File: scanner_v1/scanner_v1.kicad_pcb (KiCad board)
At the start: 2 copper layers, 59.3 x 42.2 mm, 47 parts, among them J1 Conn_01x06, J2 Conn_01x03, J3 USB_B, Q1 SS8050, Q2 SS8050, Q3 2N3906, Q4 SS8050, Q5 SS8050, U1 LM321, U2 TS2431BILT, U3 LM321, U4 PIC16F84A-XXSO, U5 LM321, U6 LM321, U7 CH340E, U8 LM7805_TO220, Y1 20Mhz

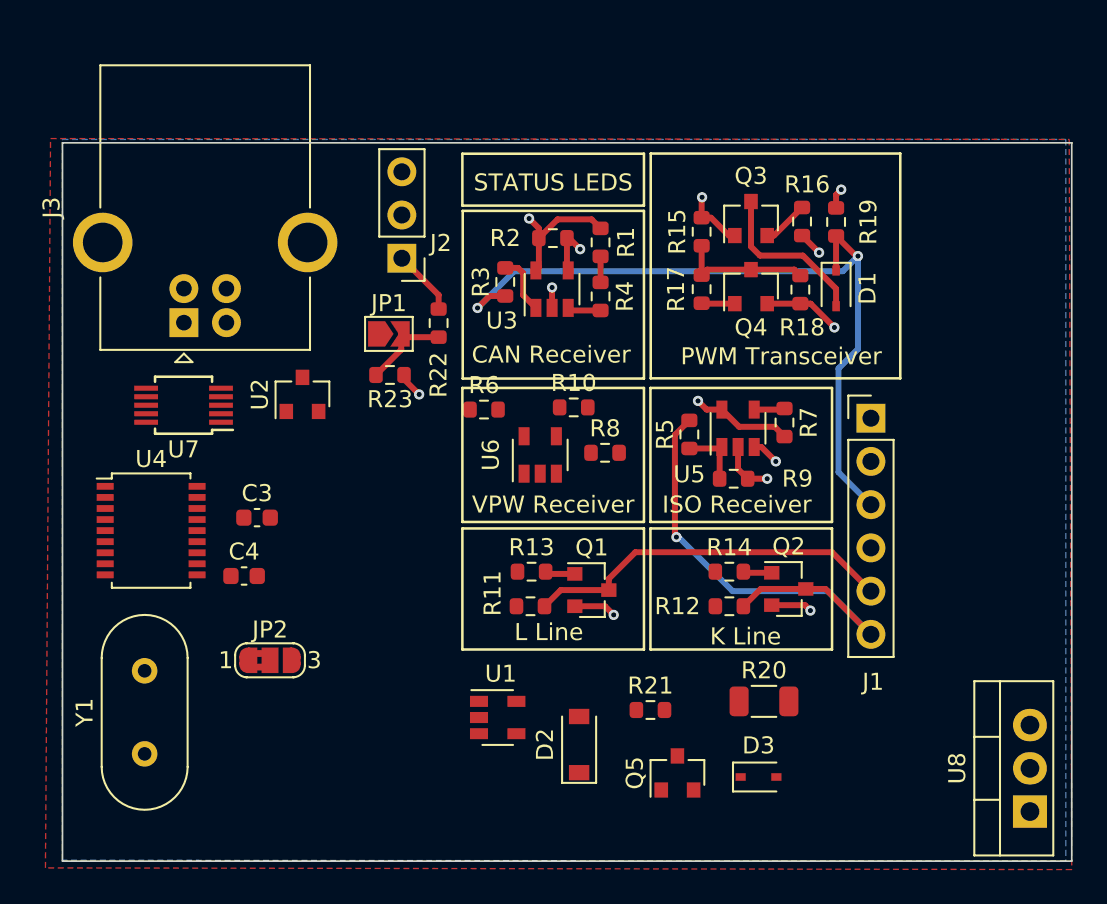
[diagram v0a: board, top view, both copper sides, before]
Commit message: finish v01
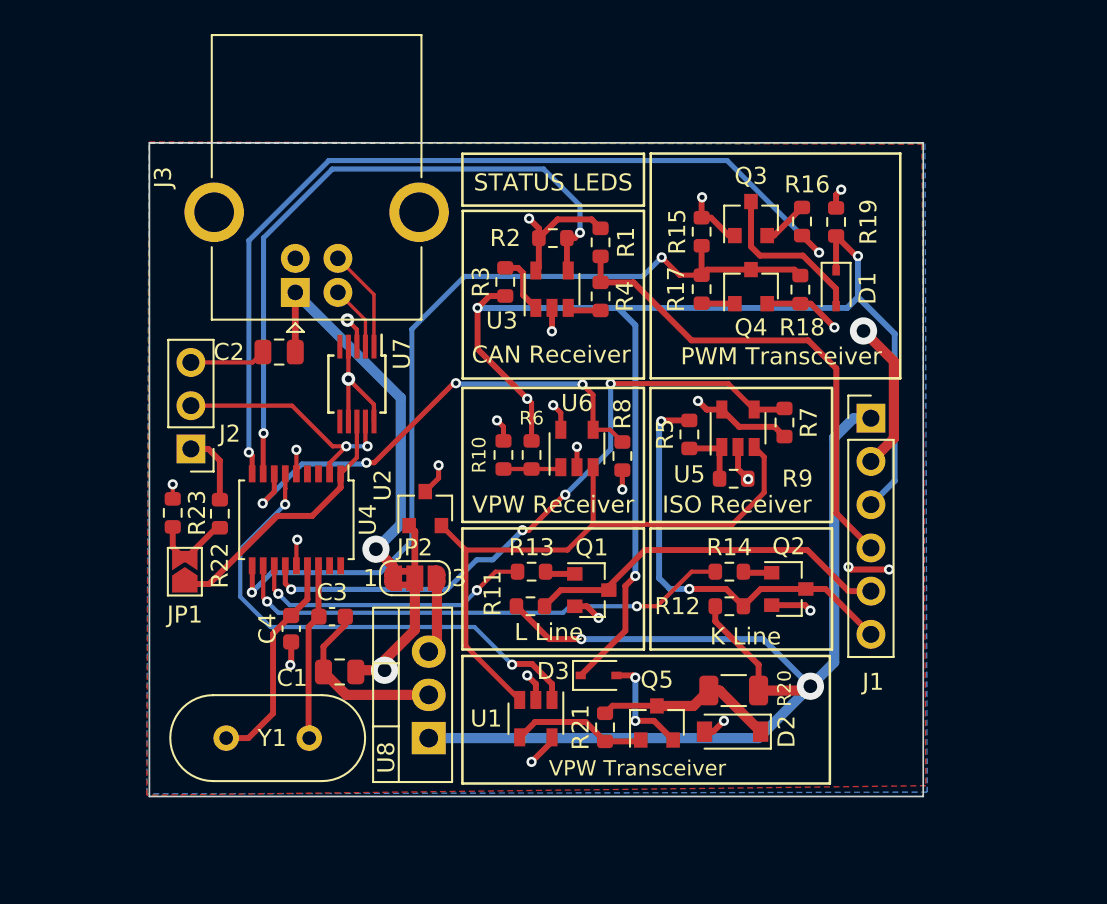
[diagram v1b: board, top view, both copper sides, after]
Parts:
- added C1: 100nF, Capacitor_SMD:C_0805_2012Metric, F.Cu at (129.2, 126.3)
- added C2: 100nF, Capacitor_SMD:C_0805_2012Metric, F.Cu at (125.6, 107.5)
- moved U8 35.6 mm to (134.4, 130.2)
- moved JP1 18.4 mm to (120.1, 120.4), turned to 90 degrees
- moved R22 17.0 mm to (122.1, 117.0)
- moved J2 16.7 mm to (120.4, 113.2)
- moved R23 15.1 mm to (119.4, 116.9), turned to -90 degrees
- moved D3 11.1 mm to (144.4, 126.5)
- moved U7 10.3 mm to (130.2, 109.4), turned to -90 degrees
- moved U2 9.85 mm to (134.2, 116.7)
- moved JP2 9.78 mm to (133.6, 120.8)
- moved D2 9.05 mm to (152.3, 129.8), turned to 180 degrees
- moved U4 8.56 mm to (126.6, 117.3), turned to -90 degrees
- moved C3 7.30 mm to (128.7, 123.0)
- moved J3 6.78 mm to (126.6, 104.0)
- moved R10 4.98 mm to (138.8, 113.5), turned to 90 degrees
- moved Y1 4.88 mm to (122.5, 130.2), turned to 0 degrees
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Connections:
- U1 pad 5: unconnected-(U1-Pad5) -> +5V
- U4 pad 7: /xVPW_T -> /xVPW_R
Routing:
- net +12V: track 0.00 -> 69.9 mm, vias 0 -> 2
- net /xCAN+: track 1.41 -> 52.9 mm, vias 1 -> 2
- net /xCAN-: track 7.81 -> 51.7 mm, vias 0 -> 2
- net /CAN+: track 45.2 -> 85.1 mm, vias 2 -> 4
- net /xISO: track 1.80 -> 38.4 mm, vias 0 -> 4
- net /xCAN: track 2.98 -> 39.5 mm, vias 1 -> 2
- net +2V5: track 1.62 -> 37.4 mm, vias 1 -> 0
- net GND: track 16.6 -> 50.2 mm, vias 7 -> 16
- net /xK_Line: track 0.00 -> 29.8 mm, vias 0 -> 2
- net /xVPW_T: track 0.00 -> 29.7 mm, vias 0 -> 2
- net /xVPW_R: track 0.00 -> 28.7 mm, vias 0 -> 4
- net +5V: track 17.2 -> 44.9 mm, vias 3 -> 11
- net /CAN-: track 1.52 -> 28.9 mm
- net /VBUS: track 0.00 -> 23.9 mm, vias 0 -> 1
- net /xL_Line: track 0.00 -> 16.9 mm, vias 0 -> 2
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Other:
- board size 59.3 x 42.2 mm -> 45.5 x 38.4 mm
- board text added: "VPW Transceiver"
